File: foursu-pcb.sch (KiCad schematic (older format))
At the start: 24 parts, among them SW1 SW_Push, U1 ATmega32U4-AU, Y1 16MHz

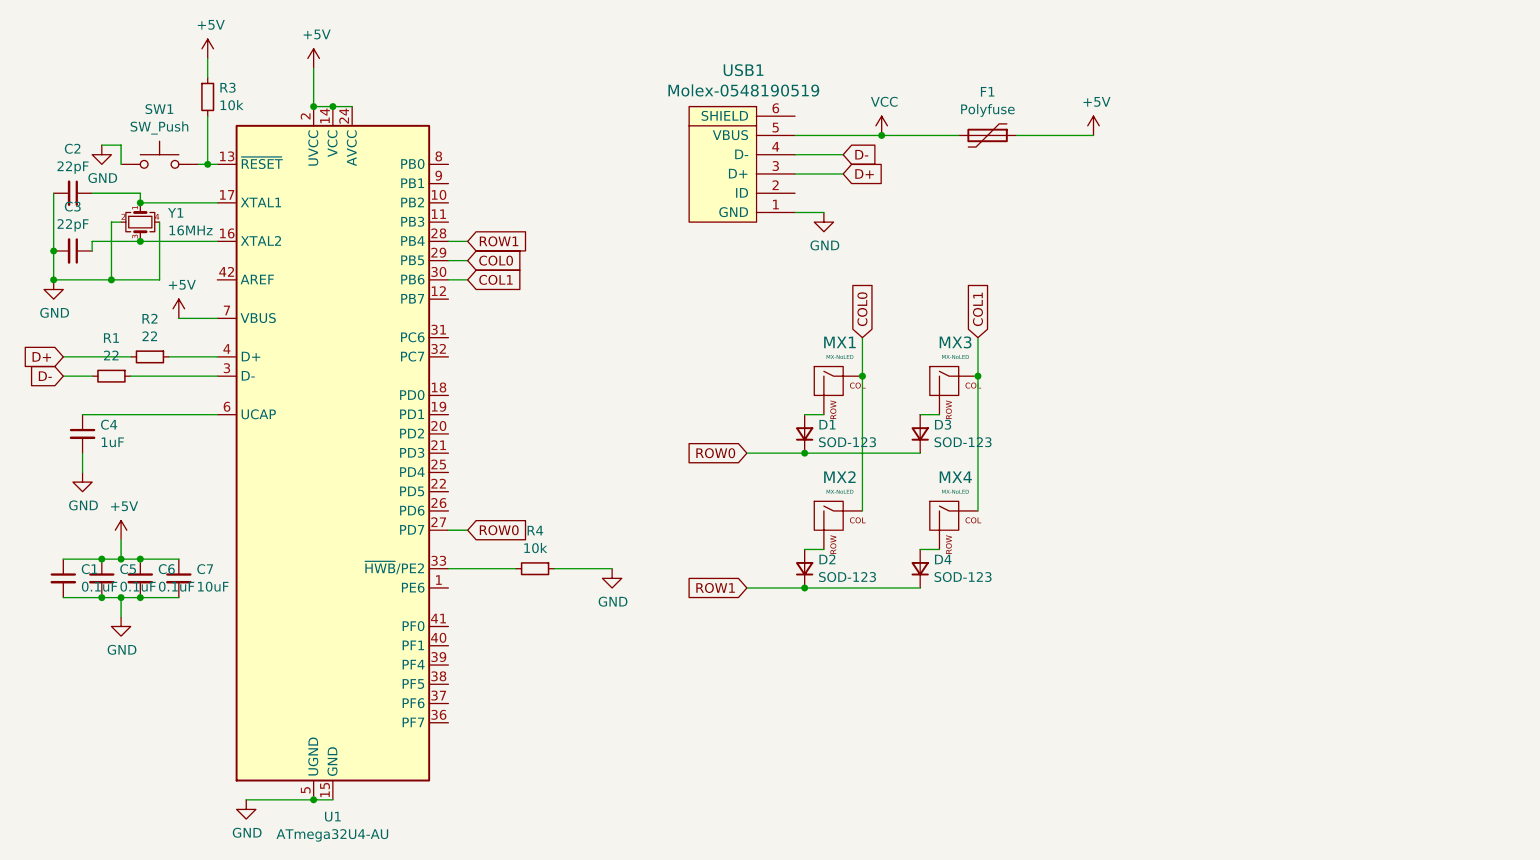
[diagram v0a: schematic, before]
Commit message: finished first prototype?
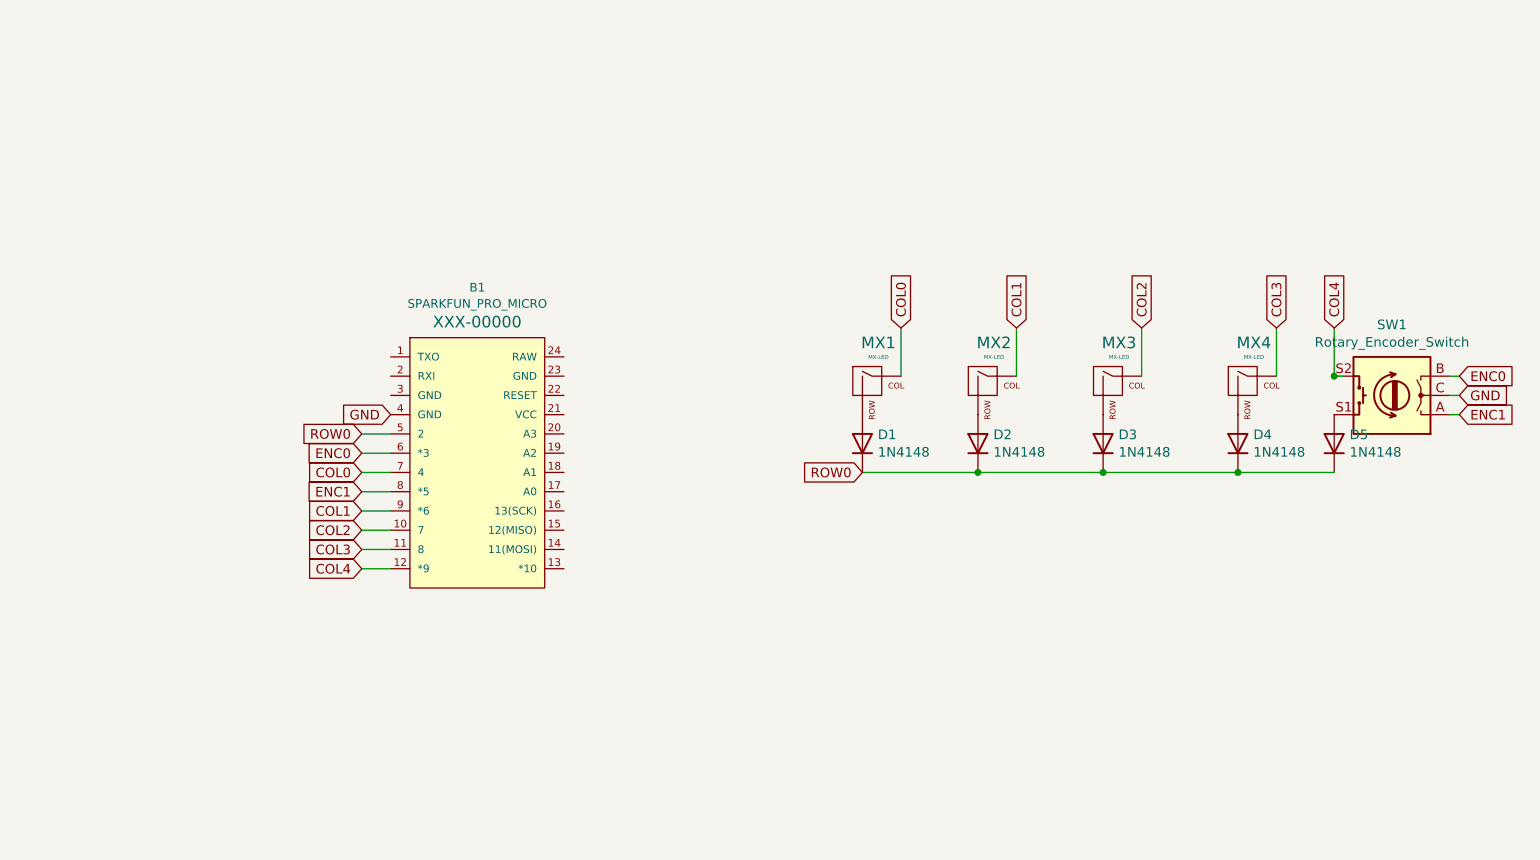
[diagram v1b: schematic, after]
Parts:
- removed C1, C5, C6: 0.1uF, Capacitor_SMD:C_0805_2012Metric, symbol Device:C_Small
- removed C2, C3: 22pF, Capacitor_SMD:C_0805_2012Metric, symbol Device:C_Small
- removed C4: 1uF, Capacitor_SMD:C_0805_2012Metric, symbol Device:C_Small
- removed C7: 10uF, Capacitor_SMD:C_0805_2012Metric, symbol Device:C_Small
- removed D1, D2, D3, D4: SOD-123, Diode_SMD:D_SOD-123, symbol Device:D_Small
- removed F1: Polyfuse, Fuse:Fuse_1206_3216Metric, symbol Device:Polyfuse
- removed R1, R2: 22, Resistor_SMD:R_0805_2012Metric, symbol Device:R_Small
- removed R3, R4: 10k, Resistor_SMD:R_0805_2012Metric, symbol Device:R_Small
- removed SW1: SW_Push, random-keyboard-parts:SKQG-1155865, symbol Switch:SW_Push
- removed U1: ATmega32U4-AU, Package_QFP:TQFP-44_10x10mm_P0.8mm, symbol MCU_Microchip_ATmega:ATmega32U4-AU
- removed USB1: Molex-0548190519, random-keyboard-parts:Molex-0548190589, symbol random-keyboard-parts:Molex-0548190519
- removed Y1: 16MHz, Crystal:Crystal_SMD_3225-4Pin_3.2x2.5mm, symbol Device:Crystal_GND24_Small
- added B1: SPARKFUN_PRO_MICRO, Boards:SPARKFUN_PRO_MICRO, symbol SparkFun-Boards:SPARKFUN_PRO_MICRO
- added D1, D2, D3, D4, D5: 1N4148, Diode_THT:D_DO-35_SOD27_P7.62mm_Horizontal, symbol Diode:1N4148
- added SW1: Rotary_Encoder_Switch, Rotary_Encoder:RotaryEncoder_Alps_EC11E-Switch_Vertical_H20mm, symbol Device:Rotary_Encoder_Switch
- MX1, MX2, MX3, MX4: value MX-NoLED -> MX-LED
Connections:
- net labels added: COL2, COL3, COL4, ENC0, ENC1
- net labels removed: +5V, D+, D-, ROW1, VCC
- wire segments 65 -> 21

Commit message: files for initial prototype
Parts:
- MX1, MX2, MX3, MX4: footprint MX_Alps_Hybrid:MX-1U-NoLED -> MX_Only:MXOnly-1U-NoLED
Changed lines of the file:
@@
 F 0 "MX1" H 5983 3673 60  0000 C CNN
 F 1 "MX-LED" H 5983 3599 20  0000 C CNN
-F 2 "MX_Alps_Hybrid:MX-1U-NoLED" H 5325 3425 60  0001 C CNN
+F 2 "MX_Only:MXOnly-1U-NoLED" H 5325 3425 60  0001 C CNN
 F 3 "" H 5325 3425 60  0001 C CNN
 	1    5950 3450
@@
 F 0 "MX2" H 6583 3673 60  0000 C CNN
 F 1 "MX-LED" H 6583 3599 20  0000 C CNN
-F 2 "MX_Alps_Hybrid:MX-1U-NoLED" H 5925 3425 60  0001 C CNN
+F 2 "MX_Only:MXOnly-1U-NoLED" H 5925 3425 60  0001 C CNN
 F 3 "" H 5925 3425 60  0001 C CNN
 	1    6550 3450
@@
 F 0 "MX3" H 7233 3673 60  0000 C CNN
 F 1 "MX-LED" H 7233 3599 20  0000 C CNN
-F 2 "MX_Alps_Hybrid:MX-1U-NoLED" H 6575 3425 60  0001 C CNN
+F 2 "MX_Only:MXOnly-1U-NoLED" H 6575 3425 60  0001 C CNN
 F 3 "" H 6575 3425 60  0001 C CNN
 	1    7200 3450
@@
 F 0 "MX4" H 7933 3673 60  0000 C CNN
 F 1 "MX-LED" H 7933 3599 20  0000 C CNN
-F 2 "MX_Alps_Hybrid:MX-1U-NoLED" H 7275 3425 60  0001 C CNN
+F 2 "MX_Only:MXOnly-1U-NoLED" H 7275 3425 60  0001 C CNN
 F 3 "" H 7275 3425 60  0001 C CNN
 	1    7900 3450
